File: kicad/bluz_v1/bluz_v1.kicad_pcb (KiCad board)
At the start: 2 copper layers, 24.9 x 14.9 mm, 71 parts, among them J1 USB_B_Micro, J10 Conn, J11 Conn, J12 BTAnt, J2 Conn, J3 Conn, J4 Conn, J5 Conn, J6 Conn, J7 Conn, J8 Conn, J9 Conn, M1 VibroMotor, Q1 RUM002N05, Q2 RUM002N05, SW1 SW_DPDT_x2, U1 MCP73831, U2 MCP1700, U3 TLV3201AIDCK, U4 AP3015KTR, Y1 NX1612SA-32MHz, Y2 NX1610-32.768

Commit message: изменено:      kicad/bluz_v1/bluz_v1.kicad_pcb 	изменено:      kicad/bluz_v1/bluz_v1.kicad_sch
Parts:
- L2: value 47uH -> 47uH LQH31CN470K03L
- R3: value 15k -> 10k
- R4: value 470 -> 220
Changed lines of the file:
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@@
       (effects (font (size 0.5 0.5) (thickness 0.07)))
     )
-    (fp_text value "47uH" (at 0 1.9) (layer "F.Fab")
+    (fp_text value "47uH LQH31CN470K03L" (at 0 1.9) (layer "F.Fab")
       (effects (font (size 1 1) (thickness 0.15)))
     )
@@
       (effects (font (size 0.5 0.5) (thickness 0.07)) (justify mirror))
     )
-    (fp_text value "470" (at 0 -1.17 90) (layer "B.Fab")
+    (fp_text value "220" (at 0 -1.17 90) (layer "B.Fab")
       (effects (font (size 1 1) (thickness 0.15)) (justify mirror))
     )
@@
       (effects (font (size 0.5 0.5) (thickness 0.07)) (justify mirror))
     )
-    (fp_text value "15k" (at 0 -1.17) (layer "B.Fab")
-      (effects (font (size 1 1) (thickness 0.15)) (justify mirror))
-    )
+    (fp_text value "10k" (at 0 -1.17) (layer "B.Fab")
+      (effects (font (size 1 1) (thickness 0.15)) (justify mirror))
+    )

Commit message: изменено:      kicad/bluz_v1/bluz_v1.kicad_pcb 	изменено:      kicad/bluz_v1/bluz_v1.kicad_sch
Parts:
- C16, C19: value 10u -> 22u C3216X5R1V226MTJ00E
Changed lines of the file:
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@@
       (effects (font (size 0.5 0.5) (thickness 0.07)))
     )
-    (fp_text value "10u" (at 0 1.85 90) (layer "F.Fab")
+    (fp_text value "22u C3216X5R1V226MTJ00E" (at 0 1.85 90) (layer "F.Fab")
       (effects (font (size 1 1) (thickness 0.15)))
     )
@@
       (effects (font (size 0.5 0.5) (thickness 0.07)) (justify mirror))
     )
-    (fp_text value "10u" (at 0 -1.85 90) (layer "B.Fab")
-      (effects (font (size 1 1) (thickness 0.15)) (justify mirror))
-    )
+    (fp_text value "22u C3216X5R1V226MTJ00E" (at 0 -1.85 90) (layer "B.Fab")
+      (effects (font (size 1 1) (thickness 0.15)) (justify mirror))
+    )

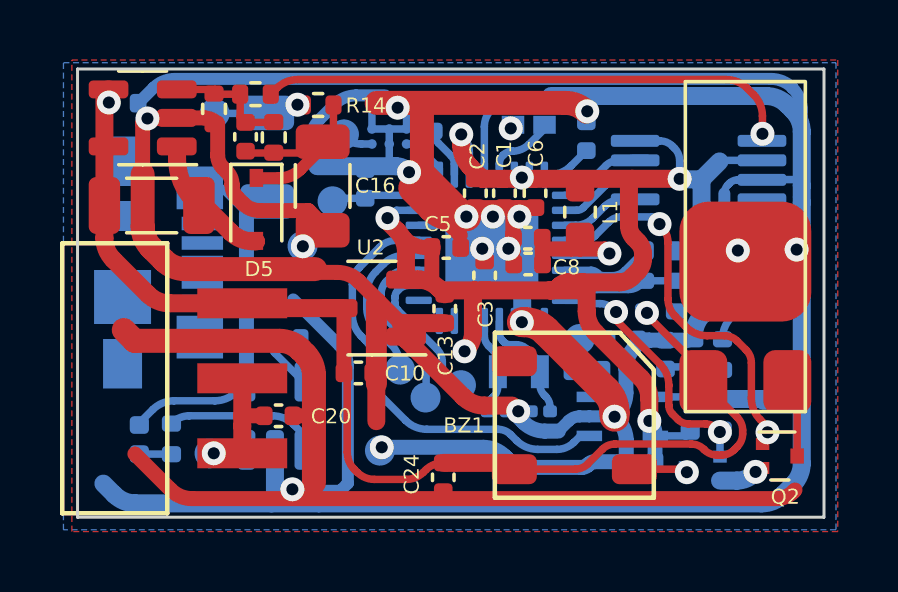
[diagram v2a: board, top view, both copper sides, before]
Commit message: изменено:      kicad/bluz_v1/bluz_v1.kicad_pcb 	изменено:      kicad/bluz_v1/bluz_v1.kicad_prl 	изменено:      kicad/bluz_v1/bluz_v1.kicad_sch 	изменено:      kicad/bluz_v1/fp-info-cache 	изменено:      stm32cubeide/BluZ_v1/.cproject 	изменено:      stm32cubeide/BluZ_v1/.settings/language.settings.xml 	изменено:      stm32cubeide/BluZ_v1/Core/Src/rw_FLASH.c 	изменено:      stm32cubeide/BluZ_v1/Debug/BluZ_v1.elf 	изменено:      stm32cubeide/BluZ_v1/Debug/BluZ_v1.hex 	изменено:      stm32cubeide/BluZ_v1/Debug/BluZ_v1.list 	изменено:      stm32cubeide/BluZ_v1/Debug/BluZ_v1.map 	изменено:      stm32cubeide/BluZ_v1/Debug/Core/Src/app_entry.d 	изменено:      stm32cubeide/BluZ_v1/Debug/Core/Src/app_entry.o 	изменено:      stm32cubeide/BluZ_v1/Debug/Core/Src/main.cyclo 	изменено:      stm32cubeide/BluZ_v1/Debug/Core/Src/main.d 	изменено:      stm32cubeide/BluZ_v1/Debug/Core/Src/main.o 	изменено:      stm32cubeide/BluZ_v1/Debug/Core/Src/main.su 	изменено:      stm32cubeide/BluZ_v1/Debug/Core/Src/stm32wbaxx_hal_msp.cyclo 	изменено:      stm32cubeide/BluZ_v1/Debug/Core/Src/stm32wbaxx_hal_msp.d 	изменено:      stm32cubeide/BluZ_v1/Debug/Core/Src/stm32wbaxx_hal_msp.o 	изменено:      stm32cubeide/BluZ_v1/Debug/Core/Src/stm32wbaxx_hal_msp.su 	изменено:      stm32cubeide/BluZ_v1/Debug/Core/Src/stm32wbaxx_it.cyclo 	изменено:      stm32cubeide/BluZ_v1/Debug/Core/Src/stm32wbaxx_it.d 	изменено:      stm32cubeide/BluZ_v1/Debug/Core/Src/stm32wbaxx_it.o 	изменено:      stm32cubeide/BluZ_v1/Debug/Core/Src/stm32wbaxx_it.su 	изменено:      stm32cubeide/BluZ_v1/Debug/Core/Src/subdir.mk 	изменено:      stm32cubeide/BluZ_v1/Debug/Core/Src/syscalls.o 	изменено:      stm32cubeide/BluZ_v1/Debug/Core/Src/sysmem.o 	изменено:      stm32cubeide/BluZ_v1/Debug/Core/Src/system_stm32wbaxx.o 	изменено:      stm32cubeide/BluZ_v1/Debug/Core/Startup/startup_stm32wba54kgux.o 	изменено:      stm32cubeide/BluZ_v1/Debug/Drivers/STM32WBAxx_HAL_Driver/Src/stm32wbaxx_hal.o 	изменено:      stm32cubeide/BluZ_v1/Debug/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
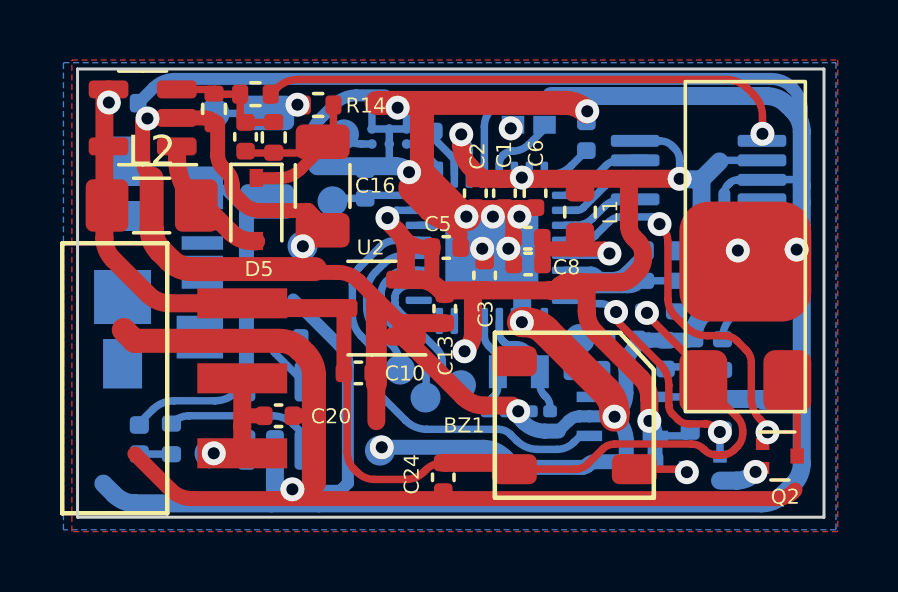
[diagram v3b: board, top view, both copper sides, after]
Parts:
- L2: footprint Inductor_SMD:L_1206_3216Metric -> Inductor_SMD:L_1206_3216Metric_Pad1.42x1.75mm_HandSolder
- R14: value 470 -> 1k
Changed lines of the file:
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@@
       (effects (font (size 0.5 0.5) (thickness 0.07)))
     )
-    (fp_text value "470" (at 0 1.17) (layer "F.Fab")
+    (fp_text value "1k" (at 0 1.17) (layer "F.Fab")
       (effects (font (size 1 1) (thickness 0.15)))
     )
@@
     )
   )
-  (footprint "Inductor_SMD:L_1206_3216Metric" (layer "F.Cu")
+  (footprint "Inductor_SMD:L_1206_3216Metric_Pad1.42x1.75mm_HandSolder" (layer "F.Cu")
     (at 64.17 41.66)
-    (descr "Inductor SMD 1206 (3216 Metric), square (rectangular) end terminal, IPC_7351 nominal, (Body size source: IPC-SM-782 page 80, https://www.pcb-3d.com/wordpress/wp-content/uploads/ipc-sm-782a_amendment_1_and_2.pdf), generated with kicad-footprint-generator")
-    (tags "inductor")
-    (property "Sheetfile" "bluz_v1.kicad_sch")
-    (property "Sheetname" "")
-    (attr smd)
-    (fp_text reference "L2" (at -0.02 -0.1) (layer "F.SilkS") hide
-      (effects (font (size 0.5 0.5) (thickness 0.07)))
-    )
-    (fp_text value "47uH LQH31CN470K03L" (at 0 1.9) (layer "F.Fab")
+    (descr "Inductor SMD 1206 (3216 Metric), square (rectangular) end terminal, IPC_7351 nominal with elongated pad for handsoldering. (Body size source: http://www.tortai-tech.com/upload/download/2011102023233369053.pdf), generated with kicad-footprint-generator")
+    (tags "inductor handsolder")
+    (property "Sheetfile" "bluz_v1.kicad_sch")
+    (property "Sheetname" "")
+    (attr smd)
+    (fp_text reference "L2" (at 0 -1.82) (layer "F.SilkS")
+      (effects (font (size 1 1) (thickness 0.15)))
+    )
+    (fp_text value "47uH LQH31CN470K03L" (at 0 1.82) (layer "F.Fab")
       (effects (font (size 1 1) (thickness 0.15)))
     )
@@
       (effects (font (size 0.8 0.8) (thickness 0.12)))
     )
-    (fp_line (start -0.835242 -0.91) (end 0.835242 -0.91) (layer "F.SilkS") (width 0.12))
-    (fp_line (start -0.835242 0.91) (end 0.835242 0.91) (layer "F.SilkS") (width 0.12))
-    (fp_line (start 2.35 1.2) (end -2.35 1.2) (layer "F.CrtYd") (width 0.05))
-    (fp_line (start -2.35 -1.2) (end 2.35 -1.2) (layer "F.CrtYd") (width 0.05))
-    (fp_line (start -2.35 1.2) (end -2.35 -1.2) (layer "F.CrtYd") (width 0.05))
-    (fp_line (start 2.35 -1.2) (end 2.35 1.2) (layer "F.CrtYd") (width 0.05))
+    (fp_line (start -0.602064 0.91) (end 0.602064 0.91) (layer "F.SilkS") (width 0.12))
+    (fp_line (start -0.602064 -0.91) (end 0.602064 -0.91) (layer "F.SilkS") (width 0.12))
+    (fp_line (start 2.45 -1.12) (end 2.45 1.12) (layer "F.CrtYd") (width 0.05))
+    (fp_line (start -2.45 1.12) (end -2.45 -1.12) (layer "F.CrtYd") (width 0.05))
+    (fp_line (start -2.45 -1.12) (end 2.45 -1.12) (layer "F.CrtYd") (width 0.05))
+    (fp_line (start 2.45 1.12) (end -2.45 1.12) (layer "F.CrtYd") (width 0.05))
+    (fp_line (start -1.6 0.8) (end -1.6 -0.8) (layer "F.Fab") (width 0.1))
+    (fp_line (start -1.6 -0.8) (end 1.6 -0.8) (layer "F.Fab") (width 0.1))
+    (fp_line (start 1.6 0.8) (end -1.6 0.8) (layer "F.Fab") (width 0.1))
     (fp_line (start 1.6 -0.8) (end 1.6 0.8) (layer "F.Fab") (width 0.1))
-    (fp_line (start -1.6 0.8) (end -1.6 -0.8) (layer "F.Fab") (width 0.1))
-    (fp_line (start 1.6 0.8) (end -1.6 0.8) (layer "F.Fab") (width 0.1))
-    (fp_line (start -1.6 -0.8) (end 1.6 -0.8) (layer "F.Fab") (width 0.1))
-    (pad "1" smd roundrect (at -1.575 0) (size 1.05 1.9) (layers "F.Cu" "F.Paste" "F.Mask") (roundrect_rratio 0.2380952381)
+    (pad "1" smd roundrect (at -1.4875 0) (size 1.425 1.75) (layers "F.Cu" "F.Paste" "F.Mask") (roundrect_rratio 0.175439)
       (net 2 "+BATT") (pinfunction "1") (pintype "passive"))
-    (pad "2" smd roundrect (at 1.575 0) (size 1.05 1.9) (layers "F.Cu" "F.Paste" "F.Mask") (roundrect_rratio 0.2380952381)
+    (pad "2" smd roundrect (at 1.4875 0) (size 1.425 1.75) (layers "F.Cu" "F.Paste" "F.Mask") (roundrect_rratio 0.175439)
       (net 39 "Net-(D5-Pad2)") (pinfunction "2") (pintype "passive"))
     (model "${KICAD6_3DMODEL_DIR}/Inductor_SMD.3dshapes/L_1206_3216Metric.wrl"
@@
   (arc (start 79.19 47.215786) (mid 79.11388 47.598469) (end 78.897107 47.922893) (width 0.25) (layer "B.Cu") (net 29))
   (segment (start 72.6475 46.03) (end 73.17 46.03) (width 0.25) (layer "F.Cu") (net 30))
+  (segment (start 63.87 38.92) (end 63.87 40.045786) (width 0.5) (layer "F.Cu") (net 30))
   (segment (start 66.335736 38.915736) (end 66.37 38.95) (width 0.5) (layer "F.Cu") (net 30))
   (segment (start 72.6475 46.1275) (end 72.6475 46.03) (width 0.6) (layer "F.Cu") (net 30))
@@
   (segment (start 71.735 44.845) (end 71.072893 44.182893) (width 0.5) (layer "F.Cu") (net 30))
   (segment (start 63.24 45.81) (end 63.6 46.17) (width 0.8) (layer "F.Cu") (net 30))
+  (segment (start 64.03 38.76) (end 63.87 38.92) (width 0.5) (layer "F.Cu") (net 30))
+  (segment (start 64.162893 40.752893) (end 64.17 40.76) (width 0.5) (layer "F.Cu") (net 30))
   (segment (start 72.47 45.58) (end 72.39 45.5) (width 0.25) (layer "F.Cu") (net 30))
-  (segment (start 64.162893 43.072893) (end 64.577107 43.487107) (width 0.8) (layer "F.Cu") (net 30))
   (segment (start 69.58 47.324214) (end 69.58 48.72) (width 0.8) (layer "F.Cu") (net 30))
   (segment (start 63.61 49.94) (end 64.807107 51.137107) (width 0.5) (layer "F.Cu") (net 30))
@@
   (segment (start 78.6 38.47) (end 78.85 38.72) (width 0.25) (layer "F.Cu") (net 30))
   (segment (start 72.39 45.5) (end 71.735 44.845) (width 0.5) (layer "F.Cu") (net 30))
-  (segment (start 63.87 40.62) (end 63.87 42.365786) (width 0.8) (layer "F.Cu") (net 30))
-  (segment (start 63.87 38.92) (end 63.87 40.62) (width 0.5) (layer "F.Cu") (net 30))
   (segment (start 68.88 48.67) (end 69.53 48.67) (width 0.5) (layer "F.Cu") (net 30))
   (segment (start 69.53 48.67) (end 69.58 48.72) (width 0.25) (layer "F.Cu") (net 30))
@@
   (segment (start 64.07 38.8) (end 64.03 38.76) (width 0.5) (layer "F.Cu") (net 30))
   (segment (start 72.91 38.24) (end 72.53 38.24) (width 0.8) (layer "F.Cu") (net 30))
+  (segment (start 64.17 42.455786) (end 64.17 40.76) (width 0.8) (layer "F.Cu") (net 30))
+  (segment (start 64.787107 43.487107) (end 64.462893 43.162893) (width 0.8) (layer "F.Cu") (net 30))
   (segment (start 76.21 43.18) (end 76.21 42.85) (width 0.5) (layer "F.Cu") (net 30))
   (segment (start 73.455 41.645) (end 74.457107 42.647107) (width 0.5) (layer "F.Cu") (net 30))
@@
   (segment (start 73.18 40.54) (end 73.18 38.51) (width 0.8) (layer "F.Cu") (net 30))
   (segment (start 74.66 42.02) (end 73.18 40.54) (width 0.8) (layer "F.Cu") (net 30))
+  (segment (start 69.62 43.78) (end 65.494214 43.78) (width 0.8) (layer "F.Cu") (net 30))
   (segment (start 65.514214 51.43) (end 69.57 51.43) (width 0.5) (layer "F.Cu") (net 30))
   (segment (start 72.8075 45.87) (end 72.6475 46.03) (width 0.25) (layer "F.Cu") (net 30))
@@
   (segment (start 83.28 44.93) (end 83.79 44.42) (width 0.25) (layer "F.Cu") (net 30))
   (segment (start 70.365786 43.89) (end 69.76 43.89) (width 0.5) (layer "F.Cu") (net 30))
-  (segment (start 64.03 38.76) (end 63.87 38.92) (width 0.5) (layer "F.Cu") (net 30))
-  (segment (start 65.284214 43.78) (end 69.62 43.78) (width 0.8) (layer "F.Cu") (net 30))
   (segment (start 72.6475 46.03) (end 72.6475 46.0375) (width 0.25) (layer "F.Cu") (net 30))
   (segment (start 69.62 43.78) (end 69.68 43.72) (width 0.5) (layer "F.Cu") (net 30))
@@
   (arc (start 66.85 40.958528) (mid 66.804328 40.728918) (end 66.674264 40.534264) (width 0.5) (layer "F.Cu") (net 30))
   (arc (start 64.807107 51.137107) (mid 65.131531 51.35388) (end 65.514214 51.43) (width 0.5) (layer "F.Cu") (net 30))
-  (arc (start 63.87 42.365786) (mid 63.94612 42.74847) (end 64.162893 43.072893) (width 0.8) (layer "F.Cu") (net 30))
   (arc (start 73.537107 41.727107) (mid 73.86153 41.94388) (end 74.244214 42.02) (width 1) (layer "F.Cu") (net 30))
+  (arc (start 64.17 42.455786) (mid 64.24612 42.838469) (end 64.462893 43.162893) (width 0.8) (layer "F.Cu") (net 30))
   (arc (start 74.557107 48.037107) (mid 74.88153 48.25388) (end 75.264214 48.33) (width 0.6) (layer "F.Cu") (net 30))
   (arc (start 71.072893 44.182893) (mid 70.74847 43.96612) (end 70.365786 43.89) (width 0.5) (layer "F.Cu") (net 30))
@@
   (arc (start 67.215686 41.595686) (mid 67.475225 41.769104) (end 67.781371 41.83) (width 0.5) (layer "F.Cu") (net 30))
   (arc (start 85.564315 51.195685) (mid 85.304776 51.369104) (end 84.998629 51.43) (width 0.5) (layer "F.Cu") (net 30))
+  (arc (start 65.494214 43.78) (mid 65.111531 43.70388) (end 64.787107 43.487107) (width 0.8) (layer "F.Cu") (net 30))
   (arc (start 76.595786 45.55) (mid 76.978469 45.62612) (end 77.302893 45.842893) (width 1) (layer "F.Cu") (net 30))
   (arc (start 79.307107 47.847107) (mid 79.52388 48.17153) (end 79.6 48.554214) (width 1) (layer "F.Cu") (net 30))
-  (arc (start 64.577107 43.487107) (mid 64.90153 43.70388) (end 65.284214 43.78) (width 0.8) (layer "F.Cu") (net 30))
   (arc (start 78.662893 38.532893) (mid 78.33847 38.31612) (end 77.955786 38.24) (width 0.8) (layer "F.Cu") (net 30))
   (arc (start 69.58 47.324214) (mid 69.50388 46.941531) (end 69.287107 46.617107) (width 0.8) (layer "F.Cu") (net 30))
   (arc (start 69.132893 46.462893) (mid 68.80847 46.24612) (end 68.425786 46.17) (width 0.8) (layer "F.Cu") (net 30))
+  (arc (start 63.87 40.045786) (mid 63.94612 40.428469) (end 64.162893 40.752893) (width 0.5) (layer "F.Cu") (net 30))
   (segment (start 79.98 50.2) (end 79.99 50.21) (width 0.25) (layer "B.Cu") (net 30))
   (segment (start 62.927107 51.297107) (end 62.56 50.93) (width 0.6) (layer "B.Cu") (net 30))

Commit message: изменено:      kicad/bluz_v1/bluz_v1.kicad_pcb 	изменено:      kicad/bluz_v1/bluz_v1.kicad_prl
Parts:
- C1, C11, C14, C2, C20, C24, C3, C5, C6: value 4.7u -> 22u
- C10, C13, C15, C23, C4, C8: value 10u -> 22u
- C18: value .1 -> 10n
- L2: value 47uH LQH31CN470K03L -> 22uH LQH31CN220K03L
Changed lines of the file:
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@@
       (effects (font (size 0.5 0.5) (thickness 0.07)))
     )
-    (fp_text value "4.7u" (at 0 1.16 90) (layer "F.Fab")
+    (fp_text value "22u" (at 0 1.16 90) (layer "F.Fab")
       (effects (font (size 1 1) (thickness 0.15)))
     )
@@
       (effects (font (size 0.5 0.5) (thickness 0.07)))
     )
-    (fp_text value "4.7u" (at 0 1.16 90) (layer "F.Fab")
+    (fp_text value "22u" (at 0 1.16 90) (layer "F.Fab")
       (effects (font (size 1 1) (thickness 0.15)))
     )
@@
       (effects (font (size 0.5 0.5) (thickness 0.07)))
     )
-    (fp_text value "4.7u" (at 0 1.16) (layer "F.Fab")
+    (fp_text value "22u" (at 0 1.16) (layer "F.Fab")
       (effects (font (size 1 1) (thickness 0.15)))
     )
@@
       (effects (font (size 0.5 0.5) (thickness 0.07)))
     )
-    (fp_text value "10u" (at 0 1.16) (layer "F.Fab")
+    (fp_text value "22u" (at 0 1.16) (layer "F.Fab")
       (effects (font (size 1 1) (thickness 0.15)))
     )
@@
       (effects (font (size 0.5 0.5) (thickness 0.07)))
     )
-    (fp_text value "4.7u" (at 0 1.16 90) (layer "F.Fab")
+    (fp_text value "22u" (at 0 1.16 90) (layer "F.Fab")
       (effects (font (size 1 1) (thickness 0.15)))
     )
@@
       (effects (font (size 0.5 0.5) (thickness 0.07)))
     )
-    (fp_text value "10u" (at 0 1.16 90) (layer "F.Fab")
+    (fp_text value "22u" (at 0 1.16 90) (layer "F.Fab")
       (effects (font (size 1 1) (thickness 0.15)))
     )
@@
       (effects (font (size 0.5 0.5) (thickness 0.07)))
     )
-    (fp_text value "4.7u" (at 0 1.16 90) (layer "F.Fab")
+    (fp_text value "22u" (at 0 1.16 90) (layer "F.Fab")
       (effects (font (size 1 1) (thickness 0.15)))
     )
@@
       (effects (font (size 0.5 0.5) (thickness 0.07)))
     )
-    (fp_text value "10u" (at 0 1.16) (layer "F.Fab")
+    (fp_text value "22u" (at 0 1.16) (layer "F.Fab")
       (effects (font (size 1 1) (thickness 0.15)))
     )
@@
       (effects (font (size 0.5 0.5) (thickness 0.07)))
     )
-    (fp_text value "4.7u" (at 0 1.16) (layer "F.Fab")
+    (fp_text value "22u" (at 0 1.16) (layer "F.Fab")
       (effects (font (size 1 1) (thickness 0.15)))
     )
@@
       (effects (font (size 0.5 0.5) (thickness 0.07)))
     )
-    (fp_text value "10u" (at 0 1.16) (layer "F.Fab")
+    (fp_text value "22u" (at 0 1.16) (layer "F.Fab")
       (effects (font (size 1 1) (thickness 0.15)))
     )
@@
       (effects (font (size 0.5 0.5) (thickness 0.07)))
     )
-    (fp_text value "4.7u" (at 0 1.16 90) (layer "F.Fab")
+    (fp_text value "22u" (at 0 1.16 90) (layer "F.Fab")
       (effects (font (size 1 1) (thickness 0.15)))
     )
@@
       (effects (font (size 1 1) (thickness 0.15)))
     )
-    (fp_text value "47uH LQH31CN470K03L" (at 0 1.82) (layer "F.Fab")
+    (fp_text value "22uH LQH31CN220K03L" (at 0 1.82) (layer "F.Fab")
       (effects (font (size 1 1) (thickness 0.15)))
     )
@@
       (effects (font (size 0.5 0.5) (thickness 0.07)) (justify mirror))
     )
-    (fp_text value "10u" (at 0 -1.16 90) (layer "B.Fab")
+    (fp_text value "22u" (at 0 -1.16 90) (layer "B.Fab")
       (effects (font (size 1 1) (thickness 0.15)) (justify mirror))
     )
@@
       (effects (font (size 0.5 0.5) (thickness 0.07)) (justify mirror))
     )
-    (fp_text value ".1" (at 0 -1.16 90) (layer "B.Fab")
+    (fp_text value "10n" (at 0 -1.16 90) (layer "B.Fab")
       (effects (font (size 1 1) (thickness 0.15)) (justify mirror))
     )
@@
       (effects (font (size 0.5 0.5) (thickness 0.07)) (justify mirror))
     )
-    (fp_text value "10u" (at 0 -1.16) (layer "B.Fab")
+    (fp_text value "22u" (at 0 -1.16) (layer "B.Fab")
       (effects (font (size 1 1) (thickness 0.15)) (justify mirror))
     )
@@
       (effects (font (size 0.5 0.5) (thickness 0.07)) (justify mirror))
     )
-    (fp_text value "4.7u" (at 0 -1.16) (layer "B.Fab")
+    (fp_text value "22u" (at 0 -1.16) (layer "B.Fab")
       (effects (font (size 1 1) (thickness 0.15)) (justify mirror))
     )
@@
       (effects (font (size 0.5 0.5) (thickness 0.07)) (justify mirror))
     )
-    (fp_text value "4.7u" (at 0 -1.16) (layer "B.Fab")
-      (effects (font (size 1 1) (thickness 0.15)) (justify mirror))
-    )
+    (fp_text value "22u" (at 0 -1.16) (layer "B.Fab")
+      (effects (font (size 1 1) (thickness 0.15)) (justify mirror))
+    )

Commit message: изменено:      kicad/bluz_v1/bluz_v1.kicad_pcb 	изменено:      kicad/bluz_v1/bluz_v1.kicad_sch
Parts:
- Y2: value NX1610-32.768 -> NX2010SA-32.768
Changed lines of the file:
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@@
       (effects (font (size 0.5 0.5) (thickness 0.07)) (justify mirror))
     )
-    (fp_text value "NX1610-32.768" (at 0 -1.8) (layer "B.Fab")
+    (fp_text value "NX2010SA-32.768" (at 0 -1.8) (layer "B.Fab")
       (effects (font (size 1 1) (thickness 0.15)) (justify mirror))
     )

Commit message: изменено:      kicad/bluz_v1/bluz_v1.kicad_pcb 	изменено:      kicad/bluz_v1/bluz_v1.kicad_sch
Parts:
- Y2: value NX2010SA-32.768 -> NX2012SA-32.768
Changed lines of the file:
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@@
       (effects (font (size 0.5 0.5) (thickness 0.07)) (justify mirror))
     )
-    (fp_text value "NX2010SA-32.768" (at 0 -1.8) (layer "B.Fab")
+    (fp_text value "NX2012SA-32.768" (at 0 -1.8) (layer "B.Fab")
       (effects (font (size 1 1) (thickness 0.15)) (justify mirror))
     )
